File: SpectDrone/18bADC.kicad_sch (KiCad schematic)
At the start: 1 part, among them U14 MCP3422A0

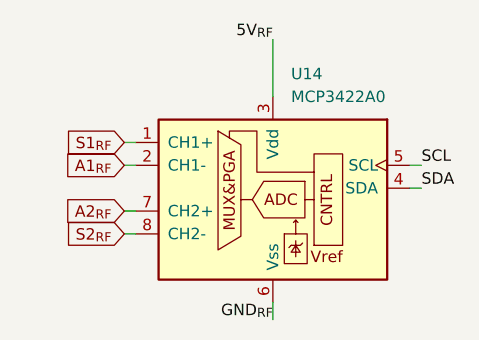
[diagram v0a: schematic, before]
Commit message: SpectDrone Development
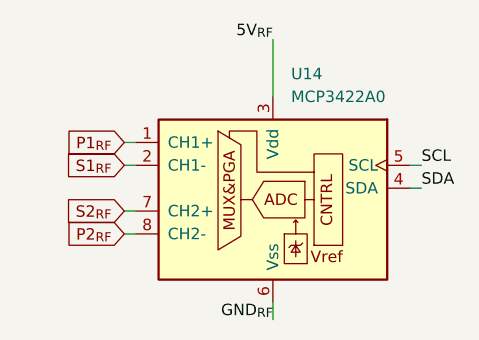
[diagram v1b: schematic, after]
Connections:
- net A1_{RF} is gone; now on net S1_{RF}: U14.2 (CH1-)
- net A2_{RF} is gone; now on net S2_{RF}: U14.7 (CH2+)
- net S1_{RF}: no longer U14.1 (CH1+)
- net S2_{RF}: no longer U14.8 (CH2-)
- new net P1_{RF}: U14.1 (CH1+)
- new net P2_{RF}: U14.8 (CH2-)
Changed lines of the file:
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@@
     (effects (font (size 1.27 1.27)) (justify right bottom))
   )
-  (global_label "S1_{RF}" (shape input) (at 98.425 86.36 180) (fields_autoplaced)
+  (global_label "P1_{RF}" (shape input) (at 98.425 86.36 180) (fields_autoplaced)
     (effects (font (size 1.27 1.27)) (justify right))
-    (property "Intersheet References" "${INTERSHEET_REFS}" (id 0) (at 91.706 86.4394 0)
+    (property "Intersheet References" "${INTERSHEET_REFS}" (id 0) (at 91.6455 86.2806 0)
       (effects (font (size 1.27 1.27)) (justify right) hide)
     )
   )
-  (global_label "S2_{RF}" (shape input) (at 98.425 96.52 180) (fields_autoplaced)
+  (global_label "P2_{RF}" (shape input) (at 98.425 96.52 180) (fields_autoplaced)
     (effects (font (size 1.27 1.27)) (justify right))
-    (property "Intersheet References" "${INTERSHEET_REFS}" (id 0) (at 91.706 96.4406 0)
+    (property "Intersheet References" "${INTERSHEET_REFS}" (id 0) (at 91.6455 96.4406 0)
       (effects (font (size 1.27 1.27)) (justify right) hide)
     )
   )
-  (global_label "A2_{RF}" (shape input) (at 98.425 93.98 180) (fields_autoplaced)
+  (global_label "S2_{RF}" (shape input) (at 98.425 93.98 180) (fields_autoplaced)
     (effects (font (size 1.27 1.27)) (justify right))
-    (property "Intersheet References" "${INTERSHEET_REFS}" (id 0) (at 91.8269 93.9006 0)
+    (property "Intersheet References" "${INTERSHEET_REFS}" (id 0) (at 91.706 93.9006 0)
       (effects (font (size 1.27 1.27)) (justify right) hide)
     )
   )
-  (global_label "A1_{RF}" (shape input) (at 98.425 88.9 180) (fields_autoplaced)
+  (global_label "S1_{RF}" (shape input) (at 98.425 88.9 180) (fields_autoplaced)
     (effects (font (size 1.27 1.27)) (justify right))
-    (property "Intersheet References" "${INTERSHEET_REFS}" (id 0) (at 91.8269 88.9794 0)
+    (property "Intersheet References" "${INTERSHEET_REFS}" (id 0) (at 91.706 88.8206 0)
       (effects (font (size 1.27 1.27)) (justify right) hide)
     )

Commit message: SpectDrone Development
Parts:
- removed U14: MCP3422A0, Package_SO:MSOP-8_3x3mm_P0.65mm, symbol Analog_ADC:MCP3422
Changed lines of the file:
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@@
 (kicad_sch (version 20211123) (generator eeschema)
   (paper "A4")
-  (wire (pts (xy 131.445 88.9) (xy 130.175 88.9))
-    (stroke (width 0) (type default) (color 0 0 0 0))
-  )
-  (wire (pts (xy 98.425 86.36) (xy 99.695 86.36))
-    (stroke (width 0) (type default) (color 0 0 0 0))
-  )
-  (wire (pts (xy 98.425 96.52) (xy 99.695 96.52))
-    (stroke (width 0) (type default) (color 0 0 0 0))
-  )
-  (wire (pts (xy 114.935 74.93) (xy 114.935 81.28))
-    (stroke (width 0) (type default) (color 0 0 0 0))
-  )
-  (wire (pts (xy 98.425 88.9) (xy 99.695 88.9))
-    (stroke (width 0) (type default) (color 0 0 0 0))
-  )
-  (wire (pts (xy 114.935 104.14) (xy 114.935 106.045))
-    (stroke (width 0) (type default) (color 0 0 0 0))
-  )
-  (wire (pts (xy 98.425 93.98) (xy 99.695 93.98))
-    (stroke (width 0) (type default) (color 0 0 0 0))
-  )
-  (wire (pts (xy 131.445 91.44) (xy 130.175 91.44))
-    (stroke (width 0) (type default) (color 0 0 0 0))
-  )
-  (label "SCL" (at 131.445 88.9 0)
-    (effects (font (size 1.27 1.27)) (justify left bottom))
-  )
-  (label "GND_{RF}" (at 114.935 106.045 180)
-    (effects (font (size 1.27 1.27)) (justify right bottom))
-  )
-  (label "SDA" (at 131.445 91.44 0)
-    (effects (font (size 1.27 1.27)) (justify left bottom))
-  )
-  (label "5V_{RF}" (at 114.935 74.93 180)
-    (effects (font (size 1.27 1.27)) (justify right bottom))
-  )
-  (global_label "P1_{RF}" (shape input) (at 98.425 86.36 180) (fields_autoplaced)
-    (effects (font (size 1.27 1.27)) (justify right))
-    (property "Intersheet References" "${INTERSHEET_REFS}" (id 0) (at 91.6455 86.2806 0)
-      (effects (font (size 1.27 1.27)) (justify right) hide)
-    )
-  )
-  (global_label "P2_{RF}" (shape input) (at 98.425 96.52 180) (fields_autoplaced)
-    (effects (font (size 1.27 1.27)) (justify right))
-    (property "Intersheet References" "${INTERSHEET_REFS}" (id 0) (at 91.6455 96.4406 0)
-      (effects (font (size 1.27 1.27)) (justify right) hide)
-    )
-  )
-  (global_label "S2_{RF}" (shape input) (at 98.425 93.98 180) (fields_autoplaced)
-    (effects (font (size 1.27 1.27)) (justify right))
-    (property "Intersheet References" "${INTERSHEET_REFS}" (id 0) (at 91.706 93.9006 0)
-      (effects (font (size 1.27 1.27)) (justify right) hide)
-    )
-  )
-  (global_label "S1_{RF}" (shape input) (at 98.425 88.9 180) (fields_autoplaced)
-    (effects (font (size 1.27 1.27)) (justify right))
-    (property "Intersheet References" "${INTERSHEET_REFS}" (id 0) (at 91.706 88.8206 0)
-      (effects (font (size 1.27 1.27)) (justify right) hide)
-    )
-  )
-  (symbol (lib_id "Analog_ADC:MCP3422") (at 114.935 91.44 0) (unit 1)
-    (in_bom yes) (on_board no) (fields_autoplaced)
-    (property "Reference" "U14" (id 0) (at 116.9544 78.74 0)
-      (effects (font (size 1.27 1.27)) (justify left))
-    )
-    (property "Value" "MCP3422A0" (id 1) (at 116.9544 81.28 0)
-      (effects (font (size 1.27 1.27)) (justify left))
-    )
-    (property "Footprint" "Package_SO:MSOP-8_3x3mm_P0.65mm" (id 2) (at 137.795 99.06 0)
-      (effects (font (size 1.27 1.27)) hide)
-    )
-    (property "Datasheet" "http://ww1.microchip.com/downloads/en/DeviceDoc/22088c.pdf" (id 3) (at 137.795 99.06 0)
-      (effects (font (size 1.27 1.27)) hide)
-    )
-    (pin "1")
-    (pin "2")
-    (pin "3")
-    (pin "4")
-    (pin "5")
-    (pin "6")
-    (pin "7")
-    (pin "8")
-  )
 )
